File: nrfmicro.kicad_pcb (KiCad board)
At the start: 2 copper layers, 18 x 33.3 mm, 24 parts, among them J1 USB_OTG, J2 USB_C_Receptacle_USB2.0, J3 Serial Connector, J4 Conn_01x02, Q1 DMG2305, SW1 SW_SPDT, U2 ProMicro, U3 AP2112K-3.3, U4 MCP73831-2-OT, U5 nRF52840, Y2 32,768

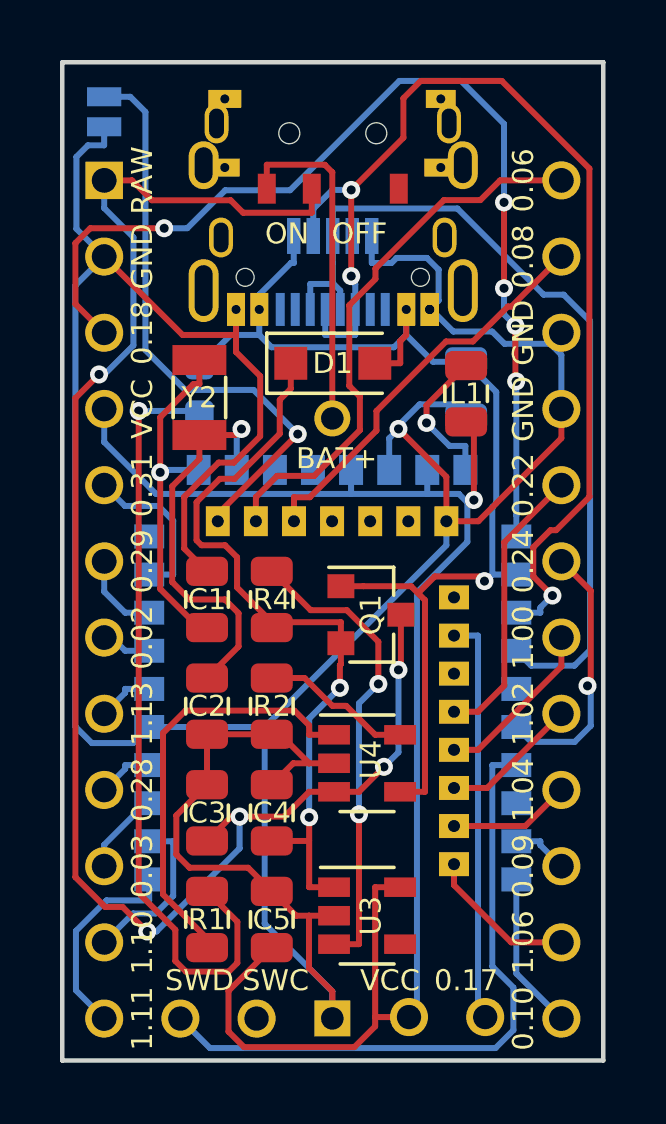
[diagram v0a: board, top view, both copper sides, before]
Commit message: pushed to version 0.2
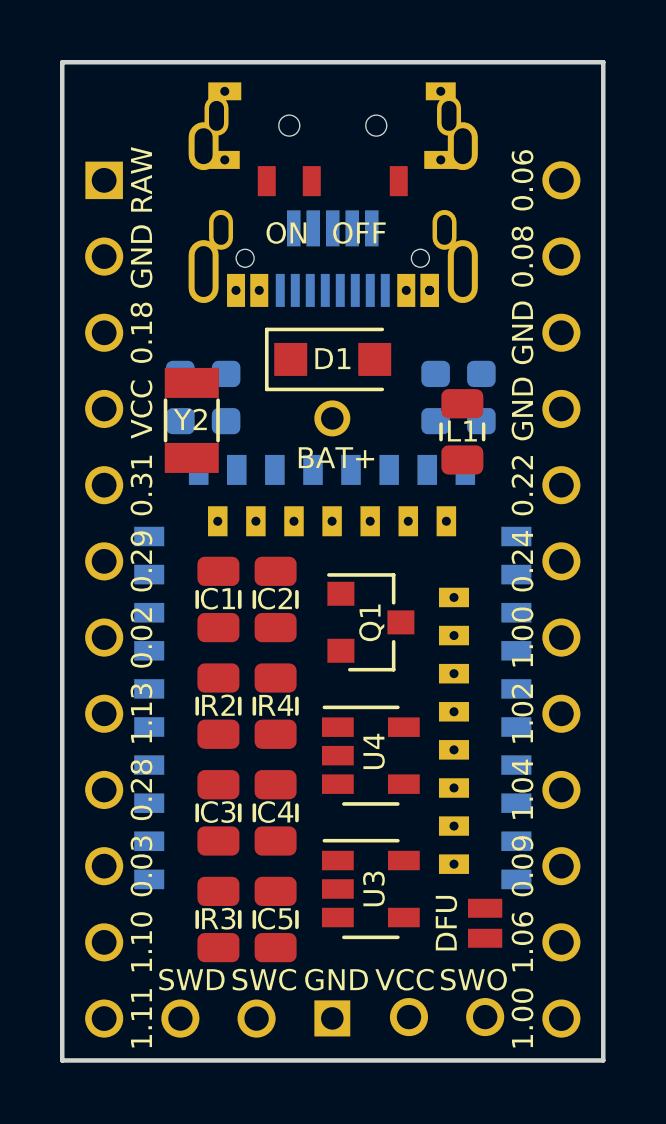
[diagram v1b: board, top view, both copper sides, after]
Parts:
- added D3: LED, LED_SMD:LED_0603_1608Metric, B.Cu at (98.7, 119.6)
- added R5: 1K, Resistor_SMD:R_0603_1608Metric, B.Cu at (100.2, 119.6)
- JP1, R3: moved to F.Cu
- R1: footprint Resistor_SMD:R_0805_2012Metric -> Resistor_SMD:R_0603_1608Metric; moved to B.Cu
- U5: value nRF52840 -> E73-2G4M08S1C-52840
- moved JP1 29.9 mm to (108.9, 137.1), turned to 180 degrees
- moved R3 19.5 mm to (100.0, 137.0)
- moved R1 19.0 mm to (107.2, 119.6)
- moved D2 9.40 mm to (108.8, 119.6), turned to 270 degrees
- moved C2 4.23 mm to (101.9, 126.3)
- moved R4 3.56 mm to (101.9, 129.9), turned to 270 degrees
- moved R2 1.78 mm to (100.0, 129.9)
- moved L1 1.28 mm to (108.1, 120.7), turned to 90 degrees
- moved U3 0.90 mm to (105.1, 136.0)
- moved Y2 0.80 mm to (99.1, 120.4), turned to 270 degrees
- moved J2 0.63 mm to (103.8, 108.5)
- moved C1 0.38 mm to (100.0, 126.3)
- moved C3 0.38 mm to (100.0, 133.4)
- moved U4 0.28 mm to (105.1, 131.5)
- moved SW1 0.25 mm to (103.8, 109.2)
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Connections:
- net MISO renamed /P0.03
- J4 pad 1: Net-(J4-Pad1) -> VBAT
- JP1 pad 1: /P0.26 -> DFU
- Q1 pad 3: VBAT -> Net-(Q1-Pad3)
- SW1 pad 3: Net-(J4-Pad1) -> Net-(Q1-Pad3)
- U2 pad 11: LED2 -> /P0.28
- U2 pad 17: SDA -> /P0.15
- U2 pad 18: SCL -> /P0.17
- U2 pad 19: /P1.00 -> /P0.20
- U2 pad 20: /P1.02 -> /P0.13
- U2 pad 21: /P1.04 -> /P0.24
- U2 pad 23: /P1.06 -> /P0.10
- U2 pad 24: /P0.10 -> /P1.06
- U2 pad 5: /P0.31 -> /P0.30
- U2 pad 6: /P0.29 -> /P0.31
- U2 pad 7: /P0.02 -> /P0.29
- U2 pad 8: /P1.13 -> /P0.02
- U2 pad 9: SCK -> /P1.13
- U5 pad 2: LED2 -> BLUE_LED
- U5 pad 30: SWO -> /P0.17
- U5 pad 34: SDA -> /P0.22
- U5 pad 35: SCL -> /P0.24
- U5 pad 36: /P1.00 -> SWO
- U5 pad 38: /P1.02 -> DFU
- U5 pad 4: SCK -> /P0.28
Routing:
- net GND: track 111.1 -> 0.00 mm, vias 1 -> 0
- net VBAT: track 53.4 -> 0.00 mm, vias 5 -> 0
- net VCC: track 52.0 -> 0.00 mm, vias 1 -> 0
- net VBUS: track 38.9 -> 0.00 mm, vias 1 -> 0
- net DATA-: track 37.5 -> 0.00 mm, vias 3 -> 0
- net RESET: track 34.4 -> 0.00 mm, vias 5 -> 0
- net DATA+: track 29.0 -> 0.00 mm
- net Net-(D2-Pad1): track 26.0 -> 0.00 mm, vias 1 -> 0
- net Net-(C4-Pad1): track 25.5 -> 0.00 mm, vias 2 -> 0
- net SWDIO: track 21.7 -> 0.00 mm
- net /P0.26: track 19.8 -> 0.00 mm, vias 1 -> 0
- net TXD: track 18.5 -> 0.00 mm
- net Net-(R4-Pad2): track 15.7 -> 0.00 mm, vias 2 -> 0
- net Net-(R1-Pad2): track 14.3 -> 0.00 mm
- net SWO: track 13.6 -> 0.00 mm
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
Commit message: updated unsaved files
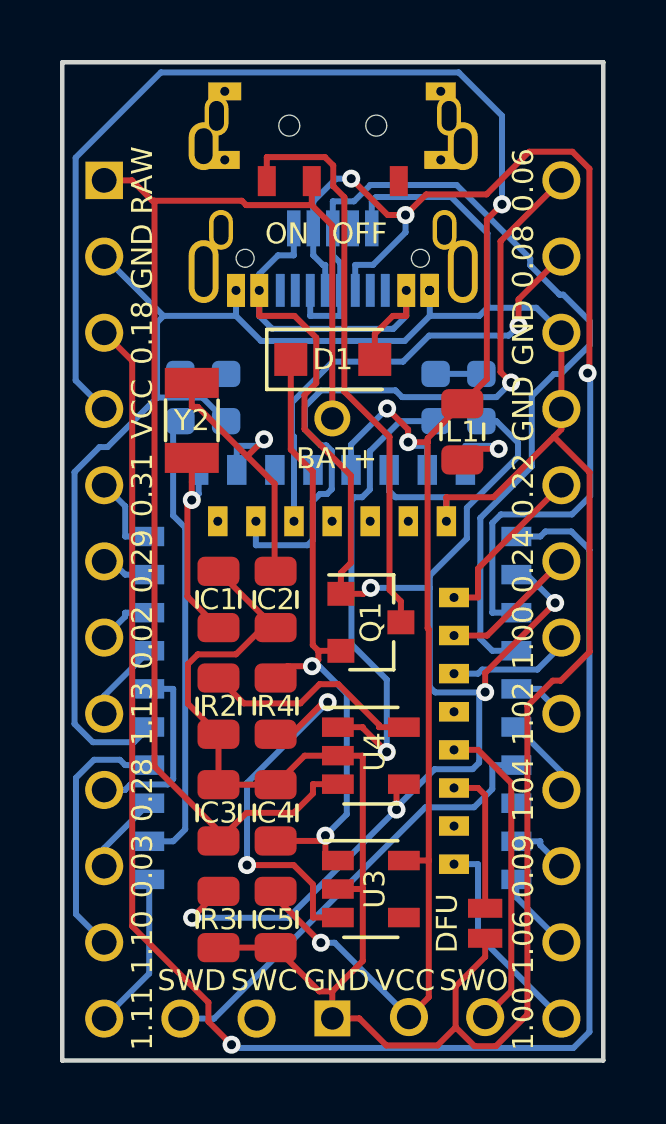
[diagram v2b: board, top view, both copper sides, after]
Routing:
- net GND: track 0.00 -> 121.5 mm
- net VCC: track 0.00 -> 69.3 mm, vias 0 -> 4
- net VBUS: track 0.00 -> 63.3 mm, vias 0 -> 5
- net RESET: track 0.00 -> 56.5 mm, vias 0 -> 1
- net VBAT: track 0.00 -> 42.5 mm
- net DATA-: track 0.00 -> 36.3 mm, vias 0 -> 3
- net DATA+: track 0.00 -> 30.2 mm
- net TXD: track 0.00 -> 23.2 mm, vias 0 -> 1
- net Net-(C4-Pad1): track 0.00 -> 22.3 mm, vias 0 -> 2
- net Net-(Q1-Pad3): track 0.00 -> 19.3 mm
- net Net-(R1-Pad2): track 0.00 -> 15.5 mm, vias 0 -> 1
- net RXD: track 0.00 -> 15.5 mm, vias 0 -> 1
- net BLUE_LED: track 0.00 -> 15.2 mm
- net SWDIO: track 0.00 -> 15.2 mm
- net Net-(R4-Pad2): track 0.00 -> 13.1 mm, vias 0 -> 2
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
